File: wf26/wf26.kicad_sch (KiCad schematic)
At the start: 7 parts, among them J1 WF26 -> TV20 S bus

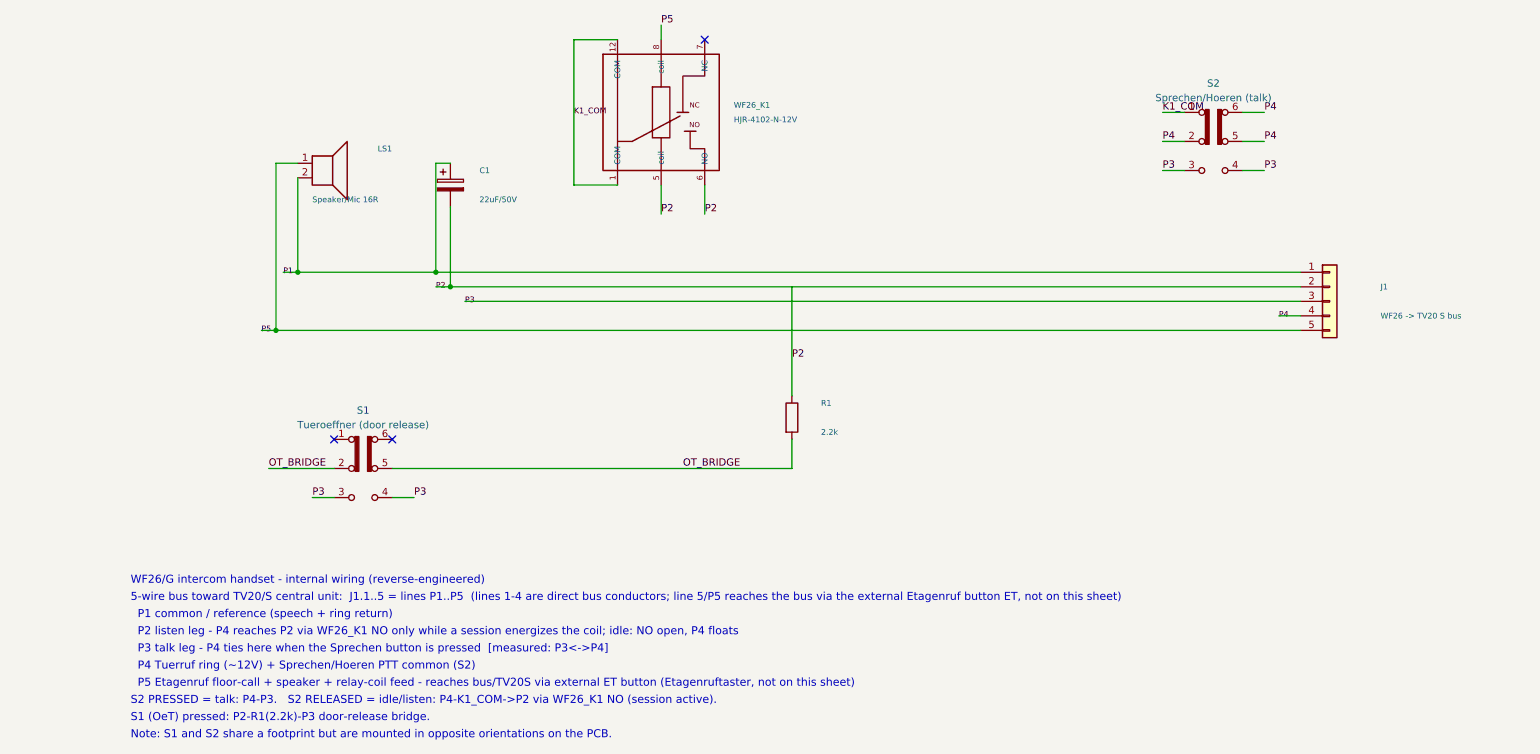
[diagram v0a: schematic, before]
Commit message: Correct WF26 internal model; rework DESIGN.md; add TODO + schematic readout
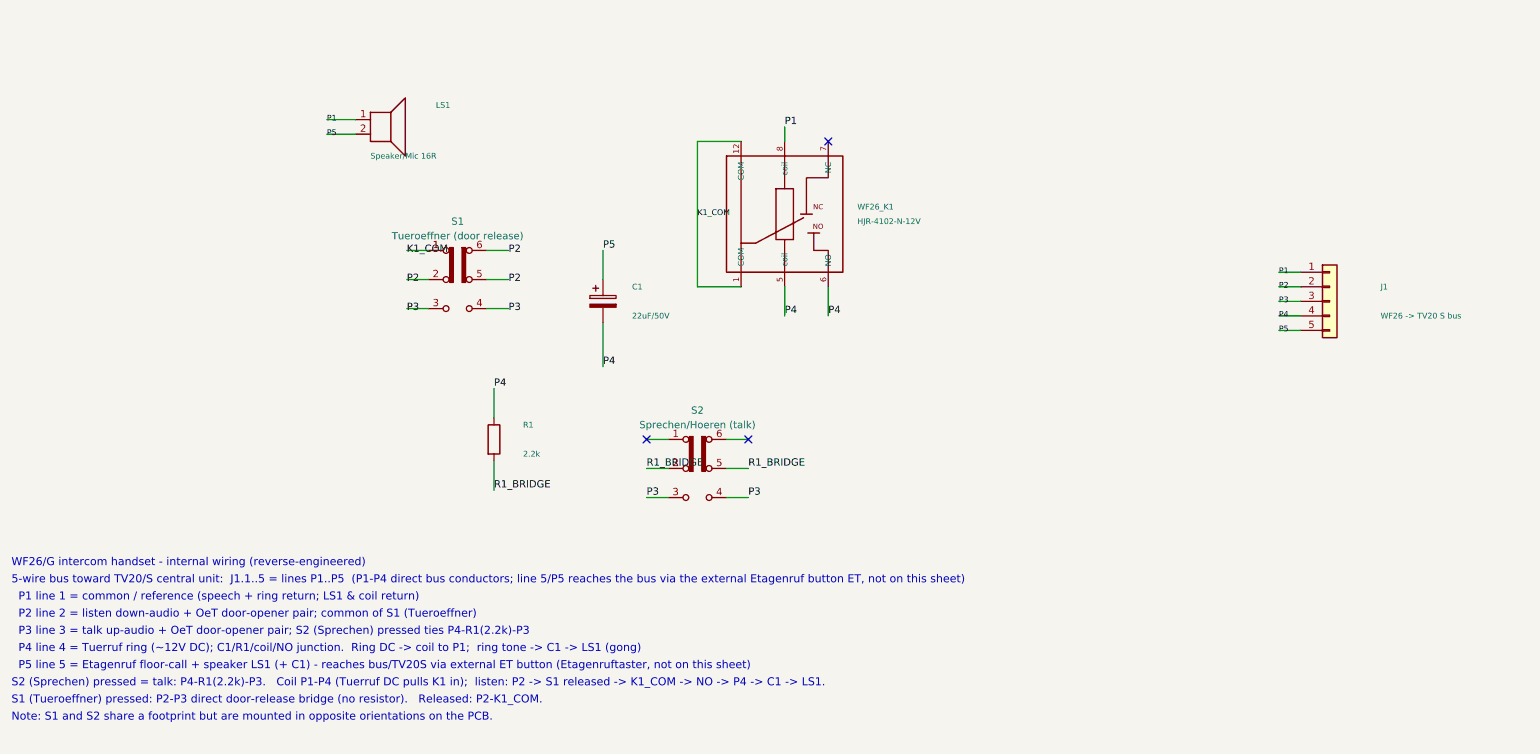
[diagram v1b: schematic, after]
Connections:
- net K1_COM: now also S1.1 (A); no longer S2.1 (A)
- net P1: now also LS1.1, WF26_K1.8 (coil); no longer C1.1, LS1.2
- net P2: now also S1.2 (B), S1.5 (B), S1.6 (C); no longer C1.2, R1.1, WF26_K1.5 (coil), WF26_K1.6 (NO)
- net P4: now also C1.2, R1.1, WF26_K1.5 (coil), WF26_K1.6 (NO); no longer S2.2 (B), S2.5 (B), S2.6 (C)
- net P5: now also C1.1, LS1.2; no longer LS1.1, WF26_K1.8 (coil)
- removed net OT_BRIDGE: R1.2, S1.2 (B), S1.5 (B)
- new net R1_BRIDGE: R1.2, S2.2 (B), S2.5 (B)
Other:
- note added: "5-wire bus toward TV20/S central unit: J1.1..5 = lines P1..P5 (P1-P4 direct bus conductors; line 5/P5 reaches the bus via the external Etagenruf button ET, not on this sheet)"
- note added: "P1 line 1 = common / reference (speech + ring return; LS1 & coil return)"
- note added: "P2 line 2 = listen down-audio + OeT door-opener pair; common of S1 (Tueroeffner)"
- note added: "P3 line 3 = talk up-audio + OeT door-opener pair; S2 (Sprechen) pressed ties P4-R1(2.2k)-P3"
- note added: "P4 line 4 = Tuerruf ring (~12V DC); C1/R1/coil/NO junction. Ring DC -> coil to P1; ring tone -> C1 -> LS1 (gong)"
- note added: "P5 line 5 = Etagenruf floor-call + speaker LS1 (+ C1) - reaches bus/TV20S via external ET button (Etagenruftaster, not on this sheet)"
- note added: "S1 (Tueroeffner) pressed: P2-P3 direct door-release bridge (no resistor). Released: P2-K1_COM."
- note added: "S2 (Sprechen) pressed = talk: P4-R1(2.2k)-P3. Coil P1-P4 (Tuerruf DC pulls K1 in); listen: P2 -> S1 released -> K1_COM -> NO -> P4 -> C1 -> LS1."
- note removed: "5-wire bus toward TV20/S central unit: J1.1..5 = lines P1..P5 (lines 1-4 are direct bus conductors; line 5/P5 reaches the bus via the external Etagenruf button ET, not on this sheet)"
- note removed: "P1 common / reference (speech + ring return)"
- note removed: "P2 listen leg - P4 reaches P2 via WF26_K1 NO only while a session energizes the coil; idle: NO open, P4 floats"
- note removed: "P3 talk leg - P4 ties here when the Sprechen button is pressed [measured: P3<->P4]"
- note removed: "P4 Tuerruf ring (~12V) + Sprechen/Hoeren PTT common (S2)"
- note removed: "P5 Etagenruf floor-call + speaker + relay-coil feed - reaches bus/TV20S via external ET button (Etagenruftaster, not on this sheet)"
- note removed: "S1 (OeT) pressed: P2-R1(2.2k)-P3 door-release bridge."
- note removed: "S2 PRESSED = talk: P4-P3. S2 RELEASED = idle/listen: P4-K1_COM->P2 via WF26_K1 NO (session active)."
- moved on the sheet: C1, LS1, R1, S1, S2, WF26_K1
